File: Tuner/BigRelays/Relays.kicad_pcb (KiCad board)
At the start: 2 copper layers, 100 x 100 mm, 93 parts, among them J1 Conn_01x03, J10 Conn_01x02, J11 Conn_01x02, J12 Conn_01x01, J13 Conn_01x01, J14 Conn_01x01, J15 Conn_01x01, J16 Conn_01x02, J17 Conn_02x10_Odd_Even, J18 Conn_01x02, J19 Conn_01x03, J2 Conn_01x03, J21 Conn_01x01, J22 Conn_01x01, J23 Conn_01x01, J24 Conn_01x01, J25 Conn_01x01, J27 Conn_01x01, J28 Conn_01x01, J29 Conn_01x01, J3 Conn_01x03, J30 Conn_01x01, J4 Conn_01x03, J5 Conn_01x03, J6 Conn_01x03, J7 Conn_01x03, J8 Conn_01x02, J9 Conn_01x02

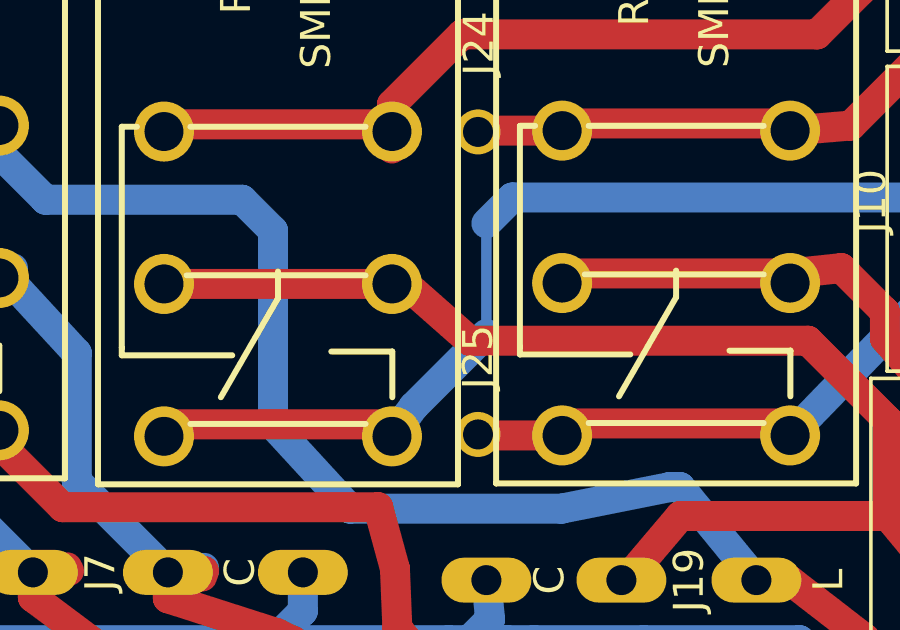
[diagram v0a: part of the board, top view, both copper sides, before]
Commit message: First code commit
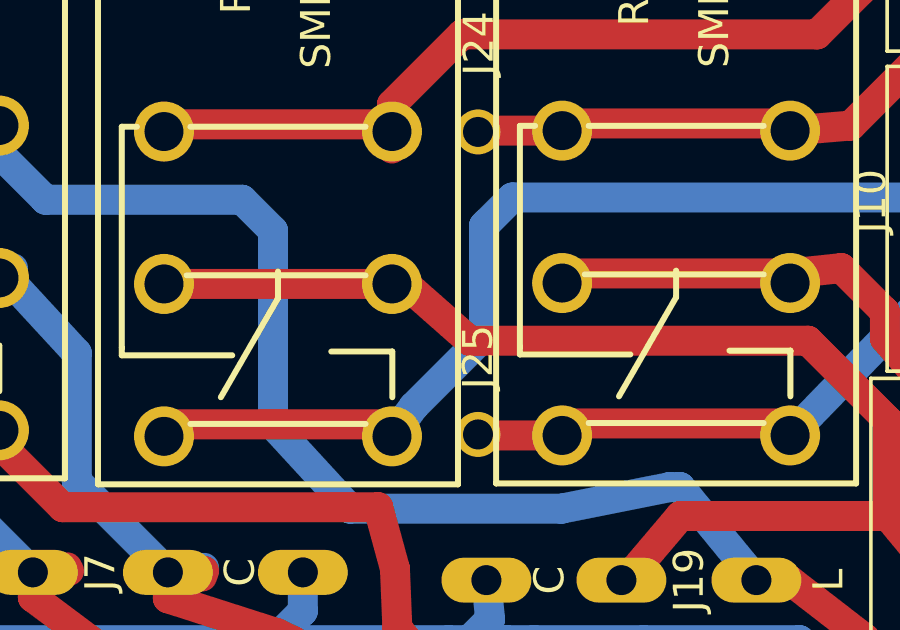
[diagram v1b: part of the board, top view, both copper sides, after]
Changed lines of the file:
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@@
     (links 292)
     (no_connects 0)
-    (area 49.924999 49.924999 150.075001 150.075001)
+    (area 44.941618 46.95878 152.967 152.888419)
     (thickness 1.6)
     (drawings 30)
-    (tracks 1023)
+    (tracks 1025)
     (zones 0)
     (modules 93)
@@
   )
   (setup
-    (last_trace_width 0.35)
+    (last_trace_width 1)
     (user_trace_width 0.35)
     (user_trace_width 0.5)
@@
   (segment (start 100.8012 79.6176) (end 103.251 82.2674) (width 1) (layer F.Cu) (net 21))
   (segment (start 103.251 82.2674) (end 109.277785 82.477785) (width 1) (layer F.Cu) (net 21))
-  (segment (start 126.8 80.2) (end 127.5212 79.2094) (width 1) (layer B.Cu) (net 22))
-  (segment (start 127.5212 79.2094) (end 129.9464 76.7842) (width 1) (layer B.Cu) (net 22))
-  (segment (start 129.9464 76.7842) (end 129.9464 73.1012) (width 0.35) (layer B.Cu) (net 22))
-  (segment (start 129.9464 73.1012) (end 130.81 72.2376) (width 1) (layer B.Cu) (net 22))
-  (segment (start 130.81 72.2376) (end 145.288 72.2376) (width 1) (layer B.Cu) (net 22))
+  (segment (start 129.86766 76.86294) (end 129.86766 73.17994) (width 1) (layer B.Cu) (net 22))
   (segment (start 145.288 72.2376) (end 147.1168 70.4088) (width 1) (layer B.Cu) (net 22))
+  (segment (start 130.81 72.2376) (end 145.288 72.2376) (width 1) (layer B.Cu) (net 22))
+  (segment (start 129.9464 73.1012) (end 130.81 72.2376) (width 1) (layer B.Cu) (net 22))
+  (segment (start 129.86766 73.17994) (end 129.9464 73.1012) (width 1) (layer B.Cu) (net 22))
+  (segment (start 126.8 80.2) (end 127.5212 79.2094) (width 1) (layer B.Cu) (net 22))
+  (segment (start 127.5212 79.2094) (end 129.86766 76.86294) (width 1) (layer B.Cu) (net 22))
+  (segment (start 129.86766 76.86294) (end 129.9464 76.7842) (width 1) (layer B.Cu) (net 22))
   (segment (start 126.8 79.8) (end 119.2 79.8) (width 1) (layer F.Cu) (net 22) (status 30))
   (segment (start 126.8 79.8) (end 126.923 79.8) (width 1) (layer B.Cu) (net 22) (status 30))
